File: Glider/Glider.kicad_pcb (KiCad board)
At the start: 2 copper layers, 100 x 200 mm, 3 parts

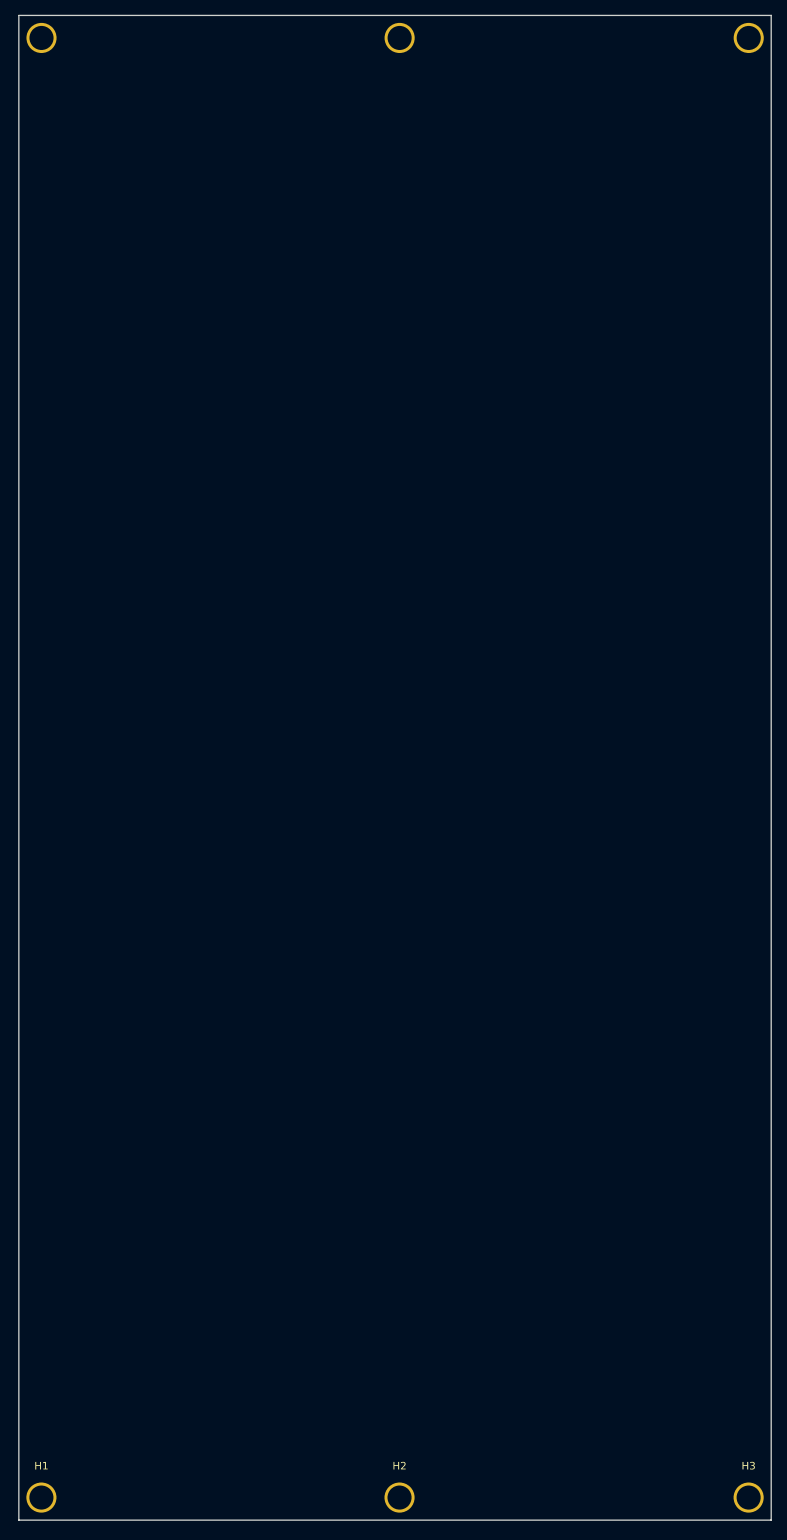
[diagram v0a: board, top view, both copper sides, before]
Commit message: Glider done !
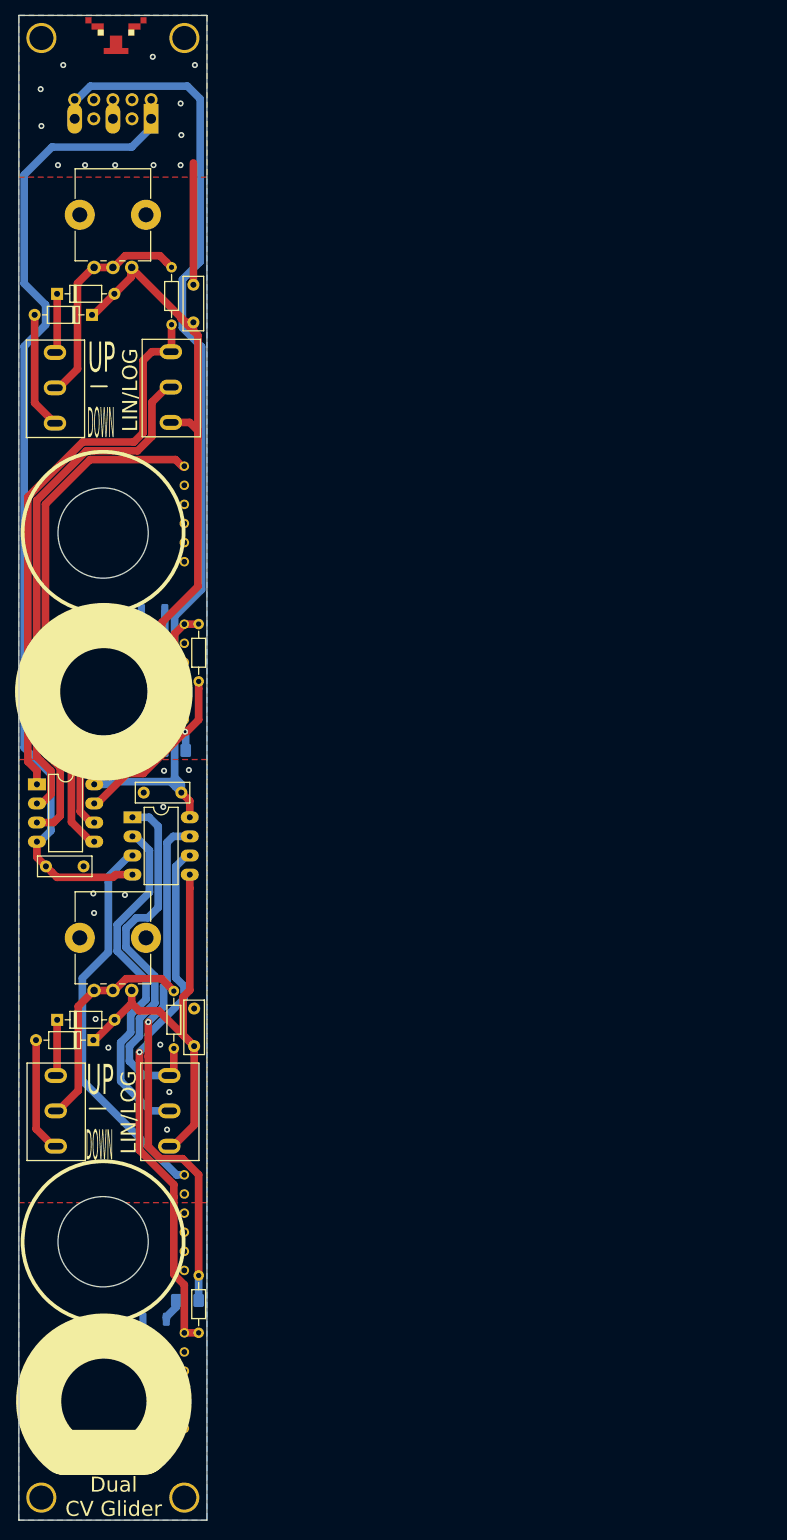
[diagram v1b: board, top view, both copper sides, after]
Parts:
- removed H3: Panel, Kosmo_panel:Kosmo_Panel_Dual_Mounting_Holes
- added C1: 100n, Capacitor_THT:C_Disc_D7.0mm_W2.5mm_P5.00mm, F.Cu at (28.7, 115.4)
- added C2: 100n, Capacitor_THT:C_Disc_D7.0mm_W2.5mm_P5.00mm, F.Cu at (20.7, 125.2)
- added C3: 470n, Capacitor_THT:C_Disc_D7.0mm_W2.5mm_P5.00mm, F.Cu at (35.3, 47.9)
- added C4: 470n, Capacitor_THT:C_Disc_D7.0mm_W2.5mm_P5.00mm, F.Cu at (35.4, 144.1)
- added D1: LED, LED_SMD:LED_1206_3216Metric_ReverseMount_Hole1.8x2.4mm, B.Cu at (29.9, 91.2)
- added D2: 1N4148, Diode_THT:D_DO-35_SOD27_P7.62mm_Horizontal, F.Cu at (21.8, 51.9)
- added D3: 1N4148, Diode_THT:D_DO-35_SOD27_P7.62mm_Horizontal, F.Cu at (17.2, 49.1)
- added D4: LED, LED_SMD:LED_1206_3216Metric_ReverseMount_Hole1.8x2.4mm, B.Cu at (30.1, 185.4)
- added D5: 1N4148, Diode_THT:D_DO-35_SOD27_P7.62mm_Horizontal, F.Cu at (22.0, 148.3)
- added D6: 1N4148, Diode_THT:D_DO-35_SOD27_P7.62mm_Horizontal, F.Cu at (17.2, 145.6)
- added J1: EuroPower, telec:EuroPower, B.Cu at (29.7, 25.8)
- added J2: OUT1, telec:JackHole, F.Cu at (23.3, 101.9)
- added J3: IN1, telec:JackHole, F.Cu at (23.3, 80.9)
- added J4: OUT2, telec:JackHole, F.Cu at (23.3, 196.1)
- added J5: IN2, telec:JackHole, F.Cu at (23.3, 175.1)
- added LOGO1: telec, logo:telec-8, F.Cu at (25.0, 16.4)
- added R1: 2k2, Resistor_SMD:R_1206_3216Metric_Pad1.42x1.75mm_HandSolder, B.Cu at (32.8, 109.8)
- added R2: 1k, Resistor_THT:R_Axial_DIN0204_L3.6mm_D1.6mm_P7.62mm_Horizontal, F.Cu at (36.0, 93.0)
- added R3: 100, Resistor_THT:R_Axial_DIN0204_L3.6mm_D1.6mm_P7.62mm_Horizontal, F.Cu at (32.4, 53.2)
- added R4: 2k2, Resistor_SMD:R_1206_3216Metric_Pad1.42x1.75mm_HandSolder, B.Cu at (34.5, 182.9)
- added R5: 1k, Resistor_THT:R_Axial_DIN0204_L3.6mm_D1.6mm_P7.62mm_Horizontal, F.Cu at (36.0, 187.2)
- added R6: 100, Resistor_THT:R_Axial_DIN0204_L3.6mm_D1.6mm_P7.62mm_Horizontal, F.Cu at (32.7, 149.4)
- added RV1: 1M, Potentiometer_THT:Potentiometer_Alps_RK09K_Single_Vertical, F.Cu at (27.1, 45.6)
- added RV2: 1M, Potentiometer_THT:Potentiometer_Alps_RK09K_Single_Vertical, F.Cu at (27.1, 141.7)
- added SW1: LIN/LOG, telec:SW_L13.2mm_W7.9mm_P4.7mm, F.Cu at (32.3, 61.5)
- added SW2: UP/DOWN, telec:SW_L13.2mm_W7.9mm_P4.7mm, F.Cu at (16.9, 61.6)
- added SW3: LIN/LOG, telec:SW_L13.2mm_W7.9mm_P4.7mm, F.Cu at (32.1, 157.7)
- added SW4: UP/DOWN, telec:SW_L13.2mm_W7.9mm_P4.7mm, F.Cu at (17.0, 157.7)
- added U1: TL082, Package_DIP:DIP-8_W7.62mm_LongPads, F.Cu at (14.5, 114.3)
- added U2: TL082, Package_DIP:DIP-8_W7.62mm_LongPads, F.Cu at (27.2, 118.7)
- H1, H2: value Panel -> Mounting_Holes
- moved H2 47.6 mm to (15.1, 209.1)
- moved H1 19.0 mm to (34.1, 209.1)
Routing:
- net -12V: track 0.00 -> 132.7 mm
- net +12V: track 0.00 -> 132.7 mm
- net Net-(C3-Pad2): track 0.00 -> 109.2 mm
- net Net-(R3-Pad1): track 0.00 -> 75.0 mm
- net Net-(J4-PadT): track 0.00 -> 71.7 mm, vias 0 -> 1
- net /OUT2: track 0.00 -> 69.4 mm, vias 0 -> 1
- net Net-(SW1-Pad2): track 0.00 -> 68.9 mm
- net /IN1: track 0.00 -> 66.8 mm
- net Net-(C4-Pad2): track 0.00 -> 58.2 mm
- net /IN2: track 0.00 -> 51.7 mm
- net Net-(R6-Pad1): track 0.00 -> 50.7 mm
- net Net-(SW3-Pad2): track 0.00 -> 46.6 mm
- net Net-(J2-PadT): track 0.00 -> 38.9 mm
- net Net-(R6-Pad2): track 0.00 -> 30.2 mm
- net Net-(R3-Pad2): track 0.00 -> 30.1 mm
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- added copper zone on B.Cu, net GND
- added copper zone on F.Cu, net GND
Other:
- board size 100 x 200 mm -> 25 x 200 mm
- board text added: "+12V"
- board text added: "-12V"
- board text added: "DOWN"
- board text added: "Dual CV Glider"
- board text added: "From Harald Antes schematic, from Ives Uson"
- board text added: "GND"
- board text added: "LIN/LOG"
- board text added: "UP"
